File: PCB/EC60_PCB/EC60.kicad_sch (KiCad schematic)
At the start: 28 parts, among them J1 JST, SW1 BOOT0, U1 STM32F401CBUx, U5 XC6206PxxxMR, Y1 8 MHz

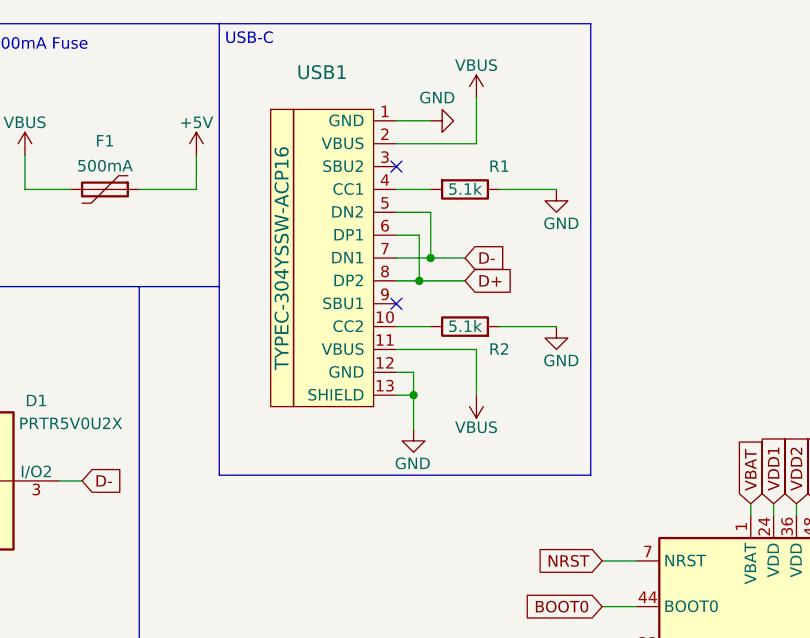
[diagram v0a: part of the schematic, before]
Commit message: cancel
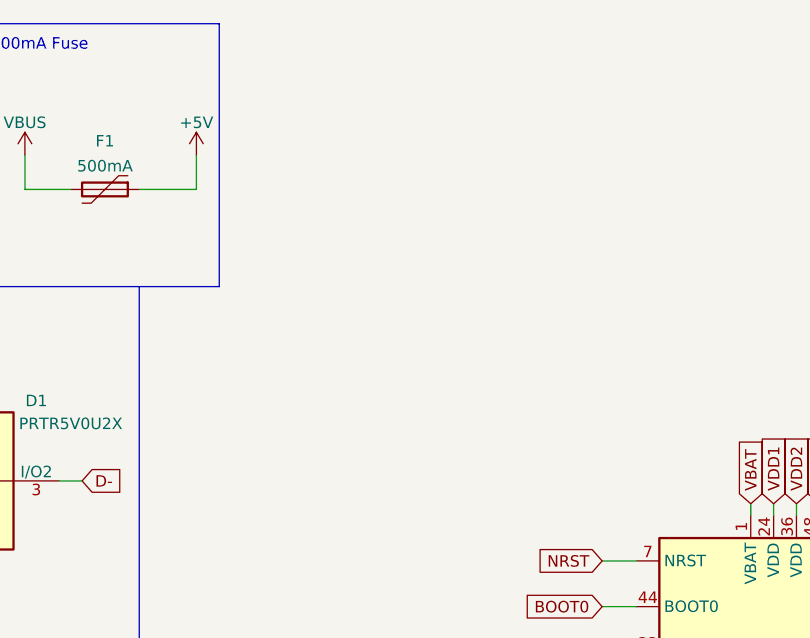
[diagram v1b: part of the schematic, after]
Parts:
- removed R1, R2: 5.1k, Resistor_SMD:R_0402_1005Metric, symbol Device:R
- removed USB1: TYPEC-304YSSW-ACP16, cipulot_parts:TYPEC-304YSSW-ACP16, symbol cipulot_parts:TYPEC-304YSSW-ACP16
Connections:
- no-connect marks 15 -> 13
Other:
- note removed: "USB-C"
